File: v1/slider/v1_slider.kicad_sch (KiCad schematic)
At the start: 0 parts

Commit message: wip
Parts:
- added C1, C3: 0.1uF, symbol Device:C
- added C2: 2.2nF, symbol Device:C
- added C4: 1uF, symbol Device:C
- added E1, E2, E3, E4, E5, E6, E7, E8: Conn_01x01, symbol Connector_Generic:Conn_01x01
- added J1: Conn_01x04, symbol Connector_Generic:Conn_01x04
- added R1, R2, R3, R4, R5, R6, R7, R8: 560, symbol Device:R
- added U1: CY8CMBR3108, Package_DFN_QFN:QFN-16-1EP_3x3mm_P0.5mm_EP1.8x1.8mm, symbol Sensor_Touch:CY8CMBR3108
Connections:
- new net: E8.1 (Pin_1), R8.1
- new net: R8.2, U1.11 (CS7)
- new net: E6.1 (Pin_1), R6.1
- new net: E4.1 (Pin_1), R4.1
- new net: R4.2, U1.13 (CS3)
- new net: E1.1 (Pin_1), R1.1
- new net: R1.2, U1.1 (CS0)
- new net: E2.1 (Pin_1), R2.1
- new net: J1.2 (Pin_2), U1.14 (SDA)
- new net: J1.3 (Pin_3), U1.15 (SCL)
- new net: E7.1 (Pin_1), R7.2
- new net: C2.1, U1.3 (CMOD)
- new net: E5.1 (Pin_1), R5.1
- new net: R5.2, U1.8 (CS4)
- new net: C1.1, U1.4 (VCC)
- new net: E3.1 (Pin_1), R3.1
- new net: R7.1, U1.10 (CS6)
- new net: R6.2, U1.9 (CS5)
- new net: R3.2, U1.12 (CS2)
- new net: R2.2, U1.2 (CS1)
- new net +5V: C3.1, C4.1, J1.4 (Pin_4), U1.5 (VDDIO), U1.6 (VDD)
- new net GND: C1.2, C2.2, C3.2, C4.2, J1.1 (Pin_1), U1.17 (EP), U1.7 (VSS)
- no-connect marks 0 -> 1

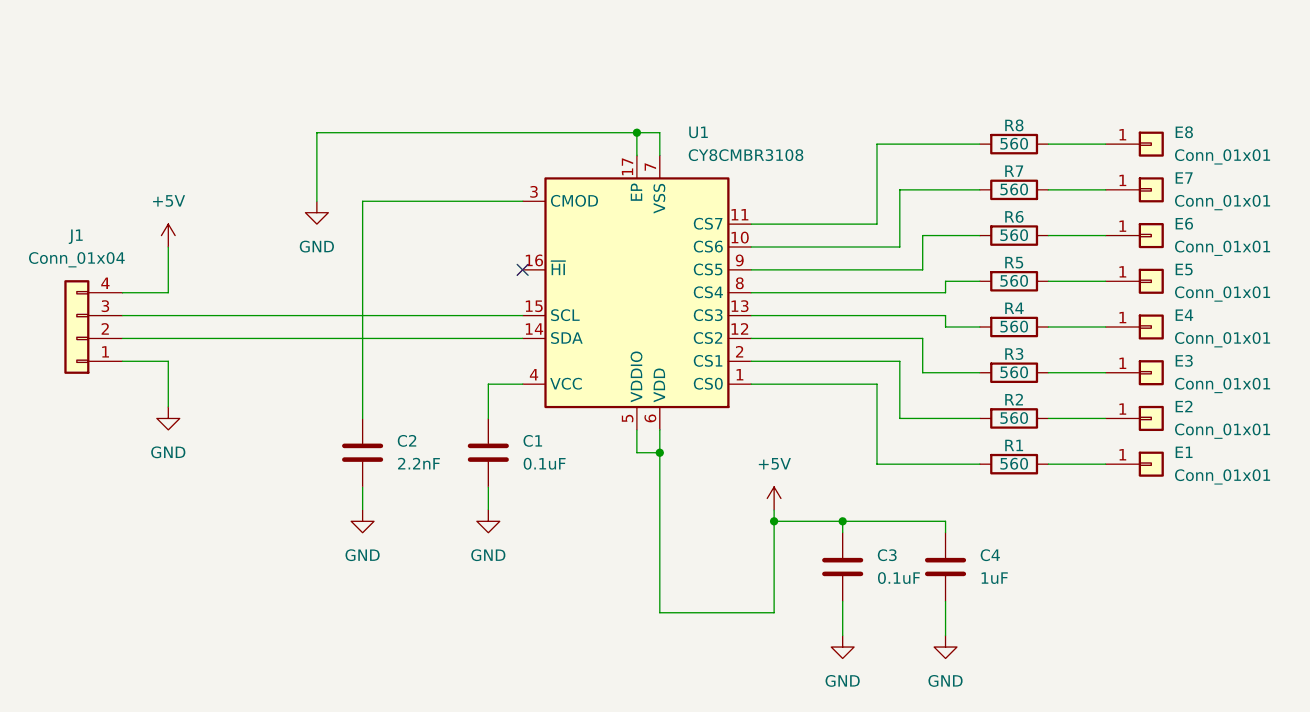
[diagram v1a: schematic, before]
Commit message: feat: impl slider sch
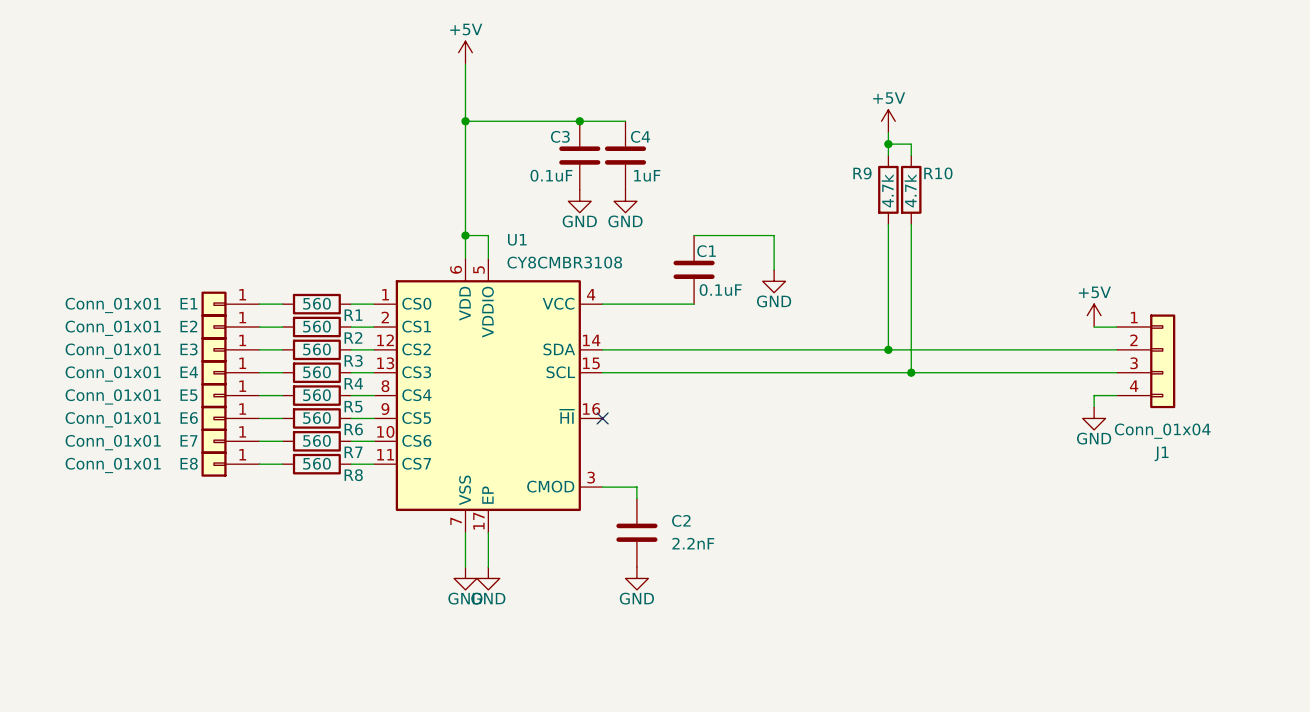
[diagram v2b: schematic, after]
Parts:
- added R10, R9: 4.7k, Resistor_SMD:R_0603_1608Metric, symbol Device:R
- C1, C2, C3, C4: footprint (none) -> Capacitor_SMD:C_0603_1608Metric
- J1: footprint (none) -> Connector_JST:JST_XH_B4B-XH-A_1x04_P2.50mm_Vertical
- R1, R2, R3, R4, R5, R6, R7, R8: footprint (none) -> Resistor_SMD:R_0603_1608Metric
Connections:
- net +5V: now also J1.1 (Pin_1), R10.1, R9.1; no longer J1.4 (Pin_4)
- net GND: now also C1.1, J1.4 (Pin_4); no longer C1.2, J1.1 (Pin_1)
- net at R8.1: now also U1.11 (CS7); no longer E8.1 (Pin_1)
- net at R8.2: now also E8.1 (Pin_1); no longer U1.11 (CS7)
- net at R6.1: now also U1.9 (CS5); no longer E6.1 (Pin_1)
- net at R4.1: now also U1.13 (CS3); no longer E4.1 (Pin_1)
- net at R4.2: now also E4.1 (Pin_1); no longer U1.13 (CS3)
- net at R1.1: now also U1.1 (CS0); no longer E1.1 (Pin_1)
- net at R1.2: now also E1.1 (Pin_1); no longer U1.1 (CS0)
- net at R2.1: now also U1.2 (CS1); no longer E2.1 (Pin_1)
- net at J1.2 (Pin_2), U1.14 (SDA): now also R9.2
- net at J1.3 (Pin_3), U1.15 (SCL): now also R10.2
- net at R5.1: now also U1.8 (CS4); no longer E5.1 (Pin_1)
- net at R5.2: now also E5.1 (Pin_1); no longer U1.8 (CS4)
- net at U1.4 (VCC): now also C1.2; no longer C1.1
- net at R3.1: now also U1.12 (CS2); no longer E3.1 (Pin_1)
- net at R6.2: now also E6.1 (Pin_1); no longer U1.9 (CS5)
- net at R3.2: now also E3.1 (Pin_1); no longer U1.12 (CS2)
- net at R2.2: now also E2.1 (Pin_1); no longer U1.2 (CS1)
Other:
- moved on the sheet: C3, C4
